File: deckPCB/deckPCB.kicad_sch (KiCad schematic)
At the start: 0 parts

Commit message: deckPCB Changes
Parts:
- added U1: RP2040, RP2040:QFN40P700X700X90-57N, symbol RP2040:RP2040
- added U2: W25Q128JVE, Package_SON:WSON-8-1EP_8x6mm_P1.27mm_EP3.4x4.3mm, symbol Memory_Flash:W25Q128JVE
- added X1, X2: DF40HC_3.0_-100DS-0.4V_58, DF40HC_3.0_-100DS-0.4V_58:HRS_DF40HC_3.0_-100DS-0.4V_58, symbol DF40HC_3.0_-100DS-0.4V_58:DF40HC_3.0_-100DS-0.4V_58
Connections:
- new net DVDD: U1.23 (DVDD), U1.50 (DVDD)
- new net IOVDD: U1.1 (IOVDD), U1.10 (IOVDD), U1.22 (IOVDD), U1.33 (IOVDD), U1.42 (IOVDD), U1.49 (IOVDD)
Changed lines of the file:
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@@
 	(generator_version "10.0")
 	(paper "A4")
-	(sheet_instances
-		(path "/"
-			(page "1")
-		)
-	)
-	(embedded_fonts no)
-)

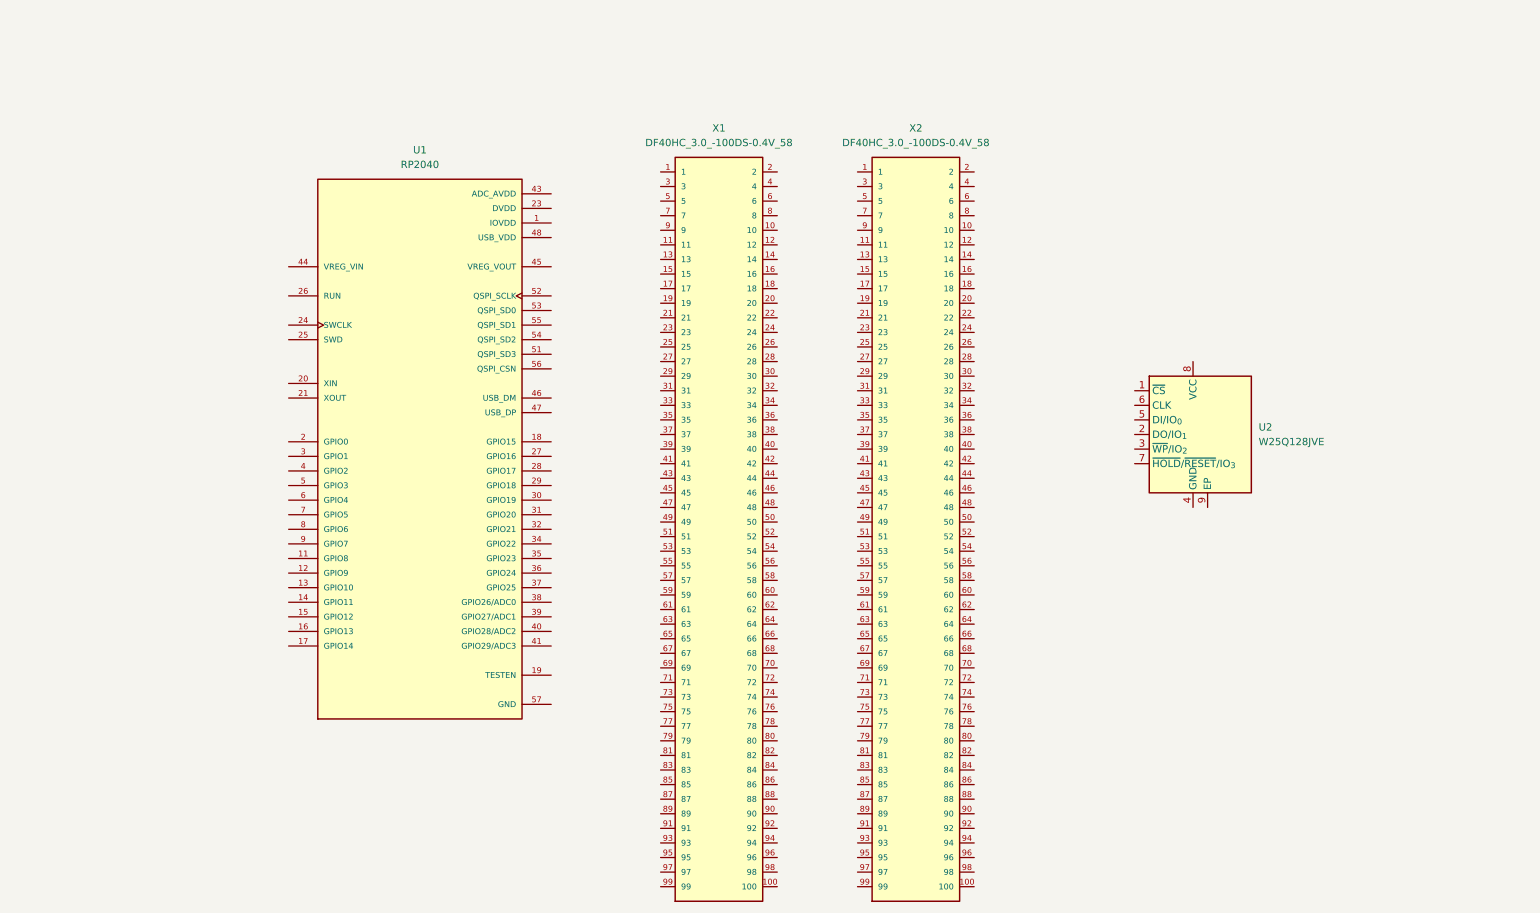
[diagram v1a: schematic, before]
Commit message: donr
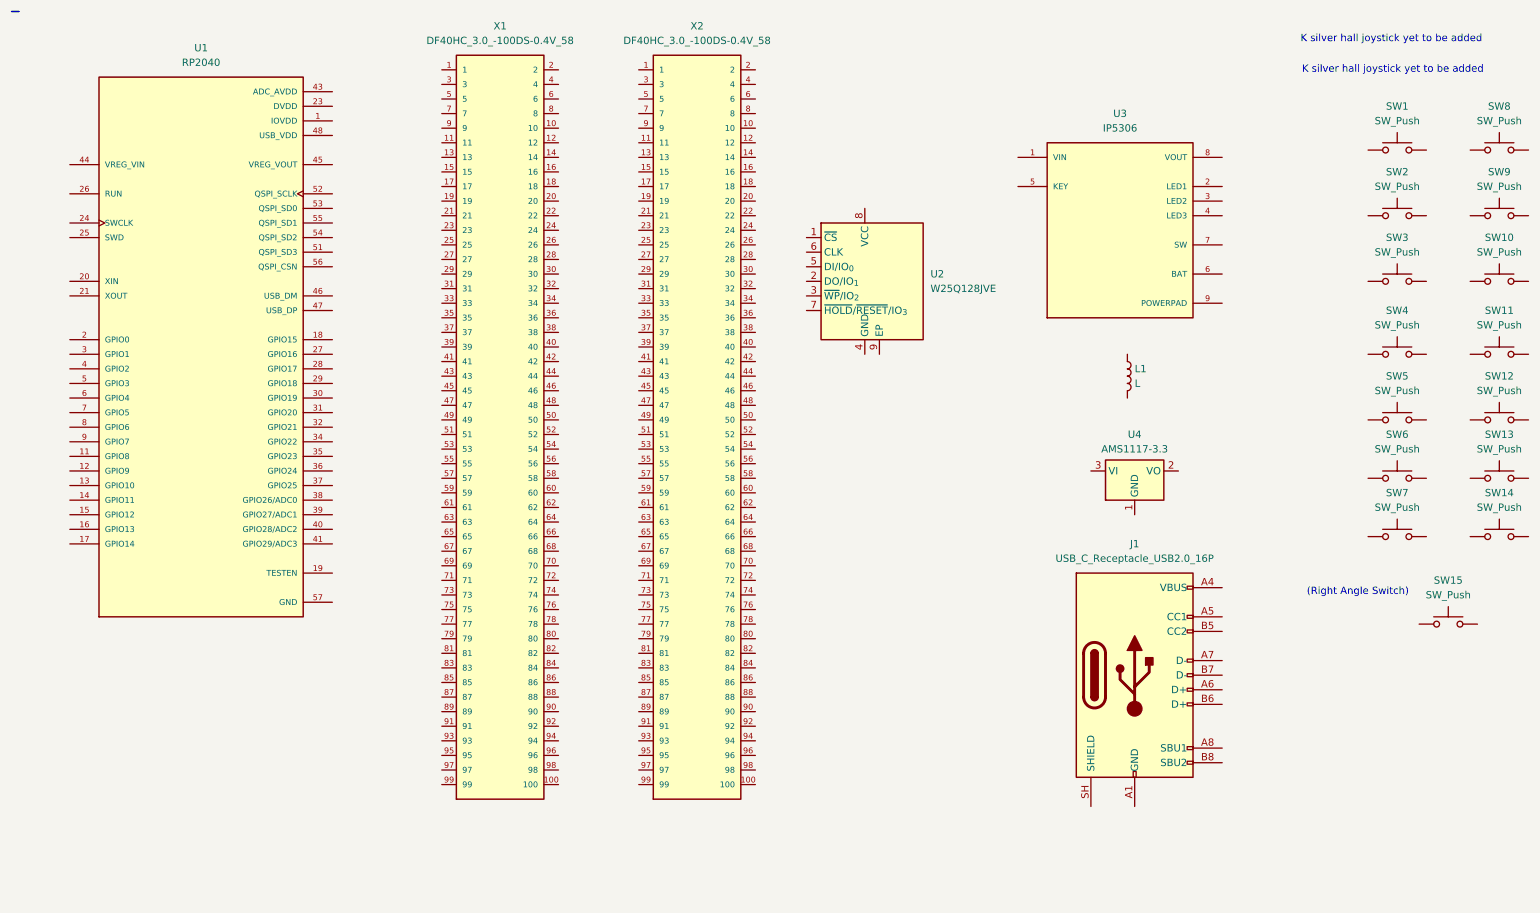
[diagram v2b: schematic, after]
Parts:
- added J1: USB_C_Receptacle_USB2.0_16P, symbol Connector:USB_C_Receptacle_USB2.0_16P
- added L1: L, symbol Device:L
- added SW1, SW10, SW11, SW12, SW13, SW14, SW15, SW2, SW3, SW4, SW5, SW6, SW7, SW8, SW9: SW_Push, symbol Switch:SW_Push
- added U3: IP5306, IP5306:SOP127P600X165-9N, symbol IP5306:IP5306
- added U4: AMS1117-3.3, Package_TO_SOT_SMD:SOT-223-3_TabPin2, symbol Regulator_Linear:AMS1117-3.3
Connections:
- new net: J1.A1 (GND), J1.A12 (GND), J1.B1 (GND), J1.B12 (GND)
- new net: J1.A4 (VBUS), J1.A9 (VBUS), J1.B4 (VBUS), J1.B9 (VBUS)
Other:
- note added: "(Right Angle Switch)"
- note added: "K silver hall joystick yet to be added"
- moved on the sheet: U1, U2, X1, X2
